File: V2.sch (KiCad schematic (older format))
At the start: 75 parts, among them J1 Input voltage, J20 Boot0, J21 Bed Temp, J22 Boot1, J26 USB_A, J27 LCD, J3 Bed Heater, J31 Bed level, J32 USB_B, J6 Head2, J7 Head1, M3 Motor Z2, M4 Motor Z1, M5 Motor Y, M6 Motor X, Q1 STN4NF20L, Q2 STN4NF20L, Q3 04N03LA, Q4 04N03LA, Q5 04N03LA, Q6 04N03LA, SW10 Button DOWN, SW11 Button UP, SW2 Boundary X, SW3 Boundary Y, SW4 Boundary Z1, SW5 Boundary Z2, SW6 Boundary E1, SW7 Boundary E2, SW8 Button BACK, SW9 Button OK, U1 LM2596S-5, U2 R-783.3-1.0, U3 STM32F105VCT6, U4 CP2104, Y1 hc49s

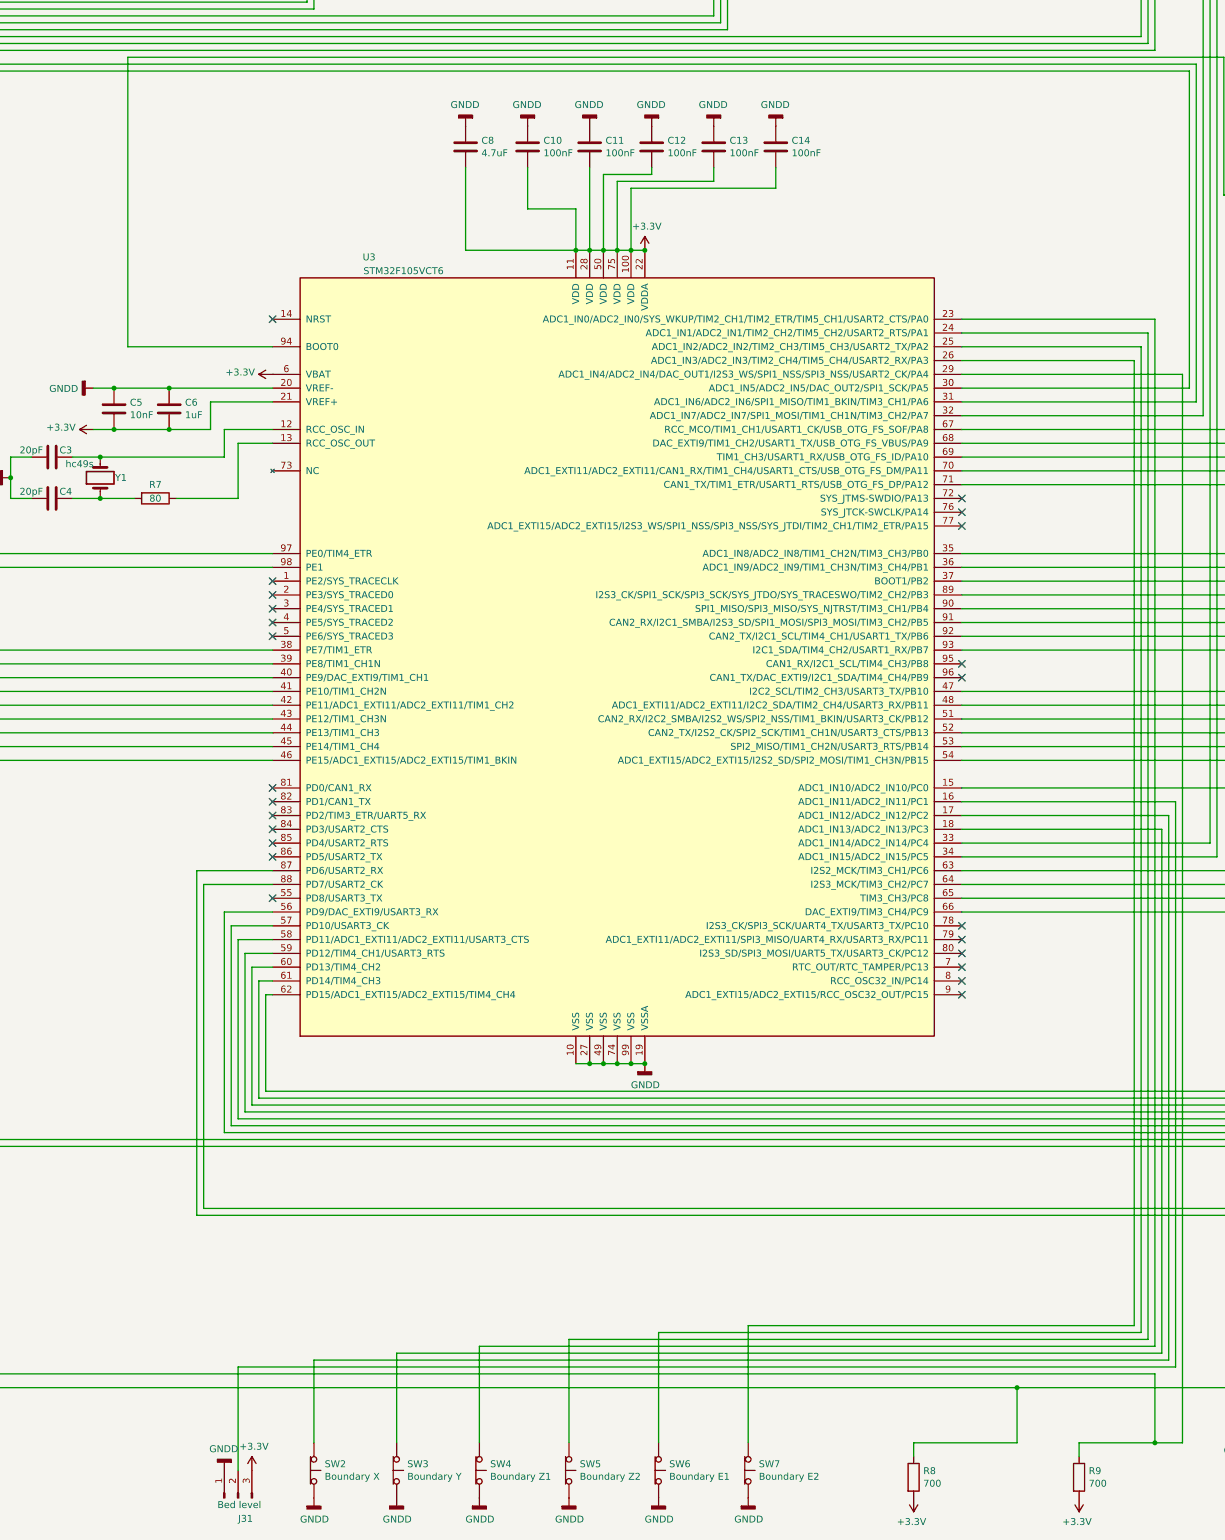
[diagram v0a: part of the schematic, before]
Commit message: Новая версия
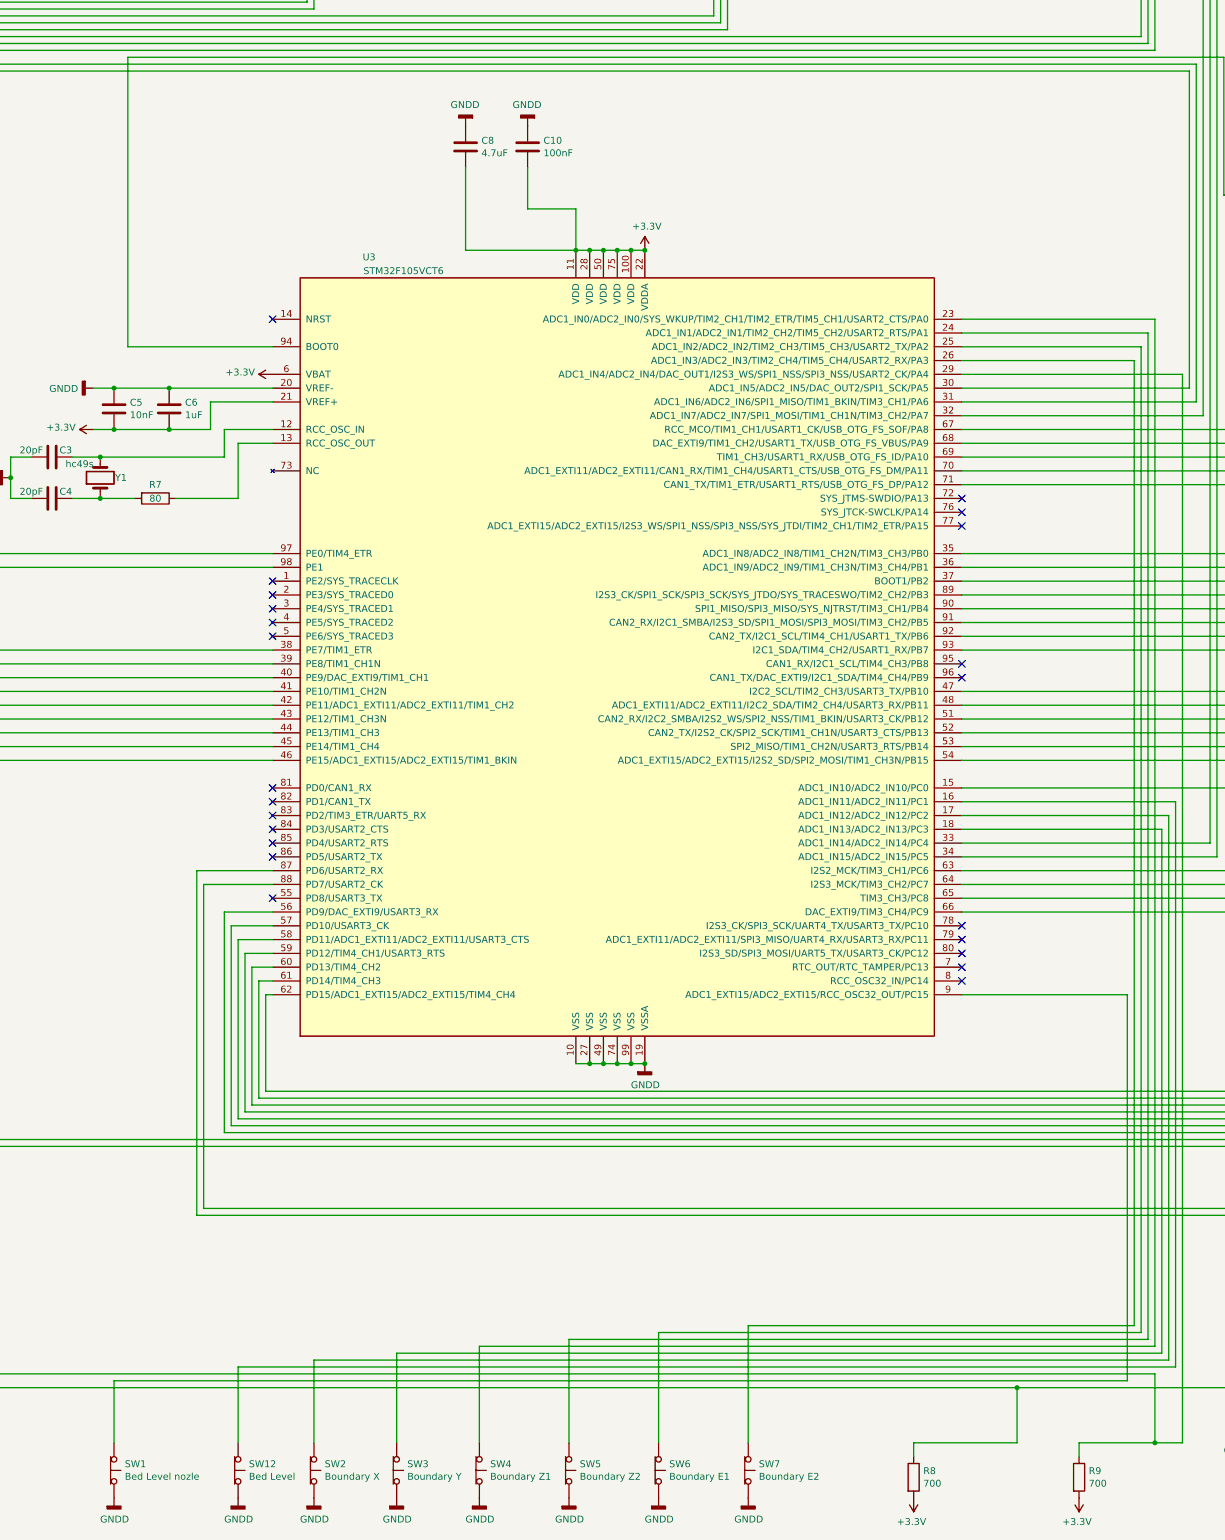
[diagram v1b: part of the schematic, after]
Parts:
- removed C11, C12, C13, C14: 100nF, Capacitor_SMD:C_1206_3216Metric, symbol V2-rescue:C-device
- removed J31: Bed level, Connector_PinHeader_2.54mm:PinHeader_1x03_P2.54mm_Vertical_SMD_Pin1Left, symbol V2-rescue:Conn_01x03_Male-Connector
- added SW1: Bed Level nozle, Connector_JST:JST_EH_B02B-EH-A_1x02_P2.50mm_Vertical, symbol V2-rescue:SW_Push_Open-Switch
- added SW12: Bed Level, Connector_JST:JST_EH_B02B-EH-A_1x02_P2.50mm_Vertical, symbol V2-rescue:SW_Push_Open-Switch
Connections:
- net GNDD: now also SW1.2 (B), SW12.2 (B)
- net at U3.16 (ADC1_IN11/ADC2_IN11/PC1): now also SW12.1 (A)
- net at U3.9 (ADC1_EXTI15/ADC2_EXTI15/RCC_OSC32_OUT/PC15): now also SW1.1 (A)
- no-connect marks 38 -> 37
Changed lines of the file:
@@
 EESchema Schematic File Version 4
 LIBS:V2-cache
-EELAYER 26 0
+EELAYER 29 0
 EELAYER END
 $Descr A2 23386 16535
@@
 $EndComp
 $Comp
-L V2-rescue:GNDD-power #PWR0130
-U 1 1 5C497D89
-P 8050 15550
-F 0 "#PWR0130" H 8050 15300 50  0001 C CNN
-F 1 "GNDD" H 8054 15395 50  0000 C CNN
-F 2 "" H 8050 15550 50  0001 C CNN
-F 3 "" H 8050 15550 50  0001 C CNN
-	1    8050 15550
-	-1   0    0    1
-$EndComp
-$Comp
 L V2-rescue:GNDD-power #PWR0131
 U 1 1 5C4985EB
@@
 	0    1    1    0
 $EndComp
-$Comp
-L V2-rescue:C-device C8
-U 1 1 5D0DBFC1
-P 9800 5950
-F 0 "C8" H 9915 5996 50  0000 L CNN
-F 1 "4.7uF" H 9915 5905 50  0000 L CNN
-F 2 "Capacitor_SMD:C_1206_3216Metric" H 9838 5800 50  0001 C CNN
-F 3 "" H 9800 5950 50  0001 C CNN
-	1    9800 5950
-	1    0    0    -1
-$EndComp
-$Comp
-L V2-rescue:GNDD-power #PWR0220
-U 1 1 5D0DC263
-P 9800 5800
-F 0 "#PWR0220" H 9800 5550 50  0001 C CNN
-F 1 "GNDD" H 9804 5645 50  0000 C CNN
-F 2 "" H 9800 5800 50  0001 C CNN
-F 3 "" H 9800 5800 50  0001 C CNN
-	1    9800 5800
-	-1   0    0    1
-$EndComp
-Wire Wire Line
-	10600 6700 10600 6400
-$Comp
-L V2-rescue:C-device C10
-U 1 1 5D18CD97
-P 10250 5950
-F 0 "C10" H 10365 5996 50  0000 L CNN
-F 1 "100nF" H 10365 5905 50  0000 L CNN
-F 2 "Capacitor_SMD:C_1206_3216Metric" H 10288 5800 50  0001 C CNN
-F 3 "" H 10250 5950 50  0001 C CNN
-	1    10250 5950
-	1    0    0    -1
-$EndComp
-$Comp
-L V2-rescue:C-device C11
-U 1 1 5D1B9492
-P 10700 5950
-F 0 "C11" H 10815 5996 50  0000 L CNN
-F 1 "100nF" H 10815 5905 50  0000 L CNN
-F 2 "Capacitor_SMD:C_1206_3216Metric" H 10738 5800 50  0001 C CNN
-F 3 "" H 10700 5950 50  0001 C CNN
-	1    10700 5950
-	1    0    0    -1
-$EndComp
-$Comp
-L V2-rescue:C-device C12
-U 1 1 5D1B9544
-P 11150 5950
-F 0 "C12" H 11265 5996 50  0000 L CNN
-F 1 "100nF" H 11265 5905 50  0000 L CNN
-F 2 "Capacitor_SMD:C_1206_3216Metric" H 11188 5800 50  0001 C CNN
-F 3 "" H 11150 5950 50  0001 C CNN
-	1    11150 5950
-	1    0    0    -1
-$EndComp
-$Comp
-L V2-rescue:C-device C13
-U 1 1 5D1B95F6
-P 11600 5950
-F 0 "C13" H 11715 5996 50  0000 L CNN
-F 1 "100nF" H 11715 5905 50  0000 L CNN
-F 2 "Capacitor_SMD:C_1206_3216Metric" H 11638 5800 50  0001 C CNN
-F 3 "" H 11600 5950 50  0001 C CNN
-	1    11600 5950
-	1    0    0    -1
-$EndComp
-$Comp
-L V2-rescue:C-device C14
-U 1 1 5D1B96B0
-P 12050 5950
-F 0 "C14" H 12165 5996 50  0000 L CNN
-F 1 "100nF" H 12165 5905 50  0000 L CNN
-F 2 "Capacitor_SMD:C_1206_3216Metric" H 12088 5800 50  0001 C CNN
-F 3 "" H 12050 5950 50  0001 C CNN
-	1    12050 5950
-	1    0    0    -1
-$EndComp
-Wire Wire Line
-	10600 6400 10250 6400
-Wire Wire Line
-	10250 6400 10250 6100
-Wire Wire Line
-	10700 6700 10700 6100
-Wire Wire Line
-	10800 6700 10800 6150
-Wire Wire Line
-	10800 6150 11150 6150
-Wire Wire Line
-	11150 6150 11150 6100
-Wire Wire Line
-	10900 6700 10900 6200
-Wire Wire Line
-	10900 6200 11600 6200
-Wire Wire Line
-	11600 6200 11600 6100
-Wire Wire Line
-	11000 6250 12050 6250
-Wire Wire Line
-	12050 6250 12050 6100
-Wire Wire Line
-	10600 6700 10700 6700
-Connection ~ 10600 6700
-Connection ~ 10700 6700
-Wire Wire Line
-	10700 6700 10800 6700
-Connection ~ 10800 6700
-Wire Wire Line
-	10800 6700 10900 6700
-Connection ~ 10900 6700
-Wire Wire Line
-	10900 6700 11000 6700
-Wire Wire Line
-	11000 6250 11000 6700
-Connection ~ 11000 6700
-Wire Wire Line
-	11000 6700 11100 6700
-Connection ~ 11100 6700
-Wire Wire Line
-	10600 6700 9800 6700
-Wire Wire Line
-	9800 6700 9800 6100
-$Comp
-L V2-rescue:GNDD-power #PWR0221
-U 1 1 5D4196BD
-P 10250 5800
-F 0 "#PWR0221" H 10250 5550 50  0001 C CNN
-F 1 "GNDD" H 10254 5645 50  0000 C CNN
-F 2 "" H 10250 5800 50  0001 C CNN
-F 3 "" H 10250 5800 50  0001 C CNN
-	1    10250 5800
-	-1   0    0    1
-$EndComp
-$Comp
-L V2-rescue:GNDD-power #PWR0222
-U 1 1 5D419762
-P 10700 5800
-F 0 "#PWR0222" H 10700 5550 50  0001 C CNN
-F 1 "GNDD" H 10704 5645 50  0000 C CNN
-F 2 "" H 10700 5800 50  0001 C CNN
-F 3 "" H 10700 5800 50  0001 C CNN
-	1    10700 5800
-	-1   0    0    1
-$EndComp
-$Comp
-L V2-rescue:GNDD-power #PWR0223
-U 1 1 5D419807
-P 11150 5800
-F 0 "#PWR0223" H 11150 5550 50  0001 C CNN
-F 1 "GNDD" H 11154 5645 50  0000 C CNN
-F 2 "" H 11150 5800 50  0001 C CNN
-F 3 "" H 11150 5800 50  0001 C CNN
-	1    11150 5800
-	-1   0    0    1
-$EndComp
-$Comp
-L V2-rescue:GNDD-power #PWR0224
-U 1 1 5D4198AC
-P 11600 5800
-F 0 "#PWR0224" H 11600 5550 50  0001 C CNN
-F 1 "GNDD" H 11604 5645 50  0000 C CNN
-F 2 "" H 11600 5800 50  0001 C CNN
-F 3 "" H 11600 5800 50  0001 C CNN
-	1    11600 5800
-	-1   0    0    1
-$EndComp
-$Comp
-L V2-rescue:GNDD-power #PWR0225
-U 1 1 5D419951
-P 12050 5800
-F 0 "#PWR0225" H 12050 5550 50  0001 C CNN
-F 1 "GNDD" H 12054 5645 50  0000 C CNN
-F 2 "" H 12050 5800 50  0001 C CNN
-F 3 "" H 12050 5800 50  0001 C CNN
-	1    12050 5800
-	-1   0    0    1
-$EndComp
 Wire Wire Line
 	10600 12600 10700 12600
@@
 	7350 7400 8400 7400
 NoConn ~ 8400 7200
-NoConn ~ 13400 12100
 Wire Wire Line
 	4300 4550 4300 4500
@@
 $EndComp
 $Comp
-L V2-rescue:Conn_01x03_Male-Connector J31
-U 1 1 5C6206CB
-P 8150 15750
-F 0 "J31" V 8000 15750 50  0000 R CNN
-F 1 "Bed level" V 8100 15900 50  0000 R CNN
-F 2 "Connector_PinHeader_2.54mm:PinHeader_1x03_P2.54mm_Vertical_SMD_Pin1Left" H 8150 15750 50  0001 C CNN
-F 3 "~" H 8150 15750 50  0001 C CNN
-	1    8150 15750
-	0    -1   -1   0
-$EndComp
-$Comp
-L V2-rescue:+3.3V-power #PWR0241
-U 1 1 5C789638
-P 8250 15550
-F 0 "#PWR0241" H 8250 15400 50  0001 C CNN
-F 1 "+3.3V" H 8265 15723 50  0000 C CNN
-F 2 "" H 8250 15550 50  0001 C CNN
-F 3 "" H 8250 15550 50  0001 C CNN
-	1    8250 15550
-	1    0    0    -1
-$EndComp
-$Comp
 L POWER_LIB:PWR_FLAG #FLG0101
 U 1 1 5C534BEB
@@
 	14950 14800 8150 14800
 Wire Wire Line
-	8150 14800 8150 15550
-Wire Wire Line
 	8700 15350 8700 14750
 Wire Wire Line
@@
 Wire Wire Line
 	14650 7500 13400 7500
+$Comp
+L V2-rescue:GNDD-power #PWR0130
+U 1 1 5C497D89
+P 8150 15750
+F 0 "#PWR0130" H 8150 15500 50  0001 C CNN
+F 1 "GNDD" H 8154 15595 50  0000 C CNN
+F 2 "" H 8150 15750 50  0001 C CNN
+F 3 "" H 8150 15750 50  0001 C CNN
+	1    8150 15750
+	1    0    0    -1
+$EndComp
+$Comp
+L V2-rescue:SW_Push_Open-Switch SW12
+U 1 1 5CFCCBD5
+P 8150 15550
+F 0 "SW12" V 8104 15628 50  0000 L CNN
+F 1 "Bed Level" V 8195 15628 50  0000 L CNN
+F 2 "Connector_JST:JST_EH_B02B-EH-A_1x02_P2.50mm_Vertical" H 8150 15750 50  0001 C CNN
+F 3 "" H 8150 15750 50  0001 C CNN
+	1    8150 15550
+	0    1    1    0
+$EndComp
+Wire Wire Line
+	8150 14800 8150 15350
+$Comp
+L V2-rescue:SW_Push_Open-Switch SW1
+U 1 1 5D0AFB29
+P 7250 15550
+F 0 "SW1" V 7204 15628 50  0000 L CNN
+F 1 "Bed Level nozle" V 7295 15628 50  0000 L CNN
+F 2 "Connector_JST:JST_EH_B02B-EH-A_1x02_P2.50mm_Vertical" H 7250 15750 50  0001 C CNN
+F 3 "" H 7250 15750 50  0001 C CNN
+	1    7250 15550
+	0    1    1    0
+$EndComp
+$Comp
+L V2-rescue:GNDD-power #PWR0114
+U 1 1 5D0B183C
+P 7250 15750
+F 0 "#PWR0114" H 7250 15500 50  0001 C CNN
+F 1 "GNDD" H 7254 15595 50  0000 C CNN
+F 2 "" H 7250 15750 50  0001 C CNN
+F 3 "" H 7250 15750 50  0001 C CNN
+	1    7250 15750
+	1    0    0    -1
+$EndComp
+Wire Wire Line
+	13400 12100 14600 12100
+Wire Wire Line
+	14600 12100 14600 14900
+Wire Wire Line
+	14600 14900 7250 14900
+Wire Wire Line
+	7250 14900 7250 15350
+Connection ~ 11100 6700
+Wire Wire Line
+	11000 6700 11100 6700
+Connection ~ 11000 6700
+Wire Wire Line
+	10900 6700 11000 6700
+Connection ~ 10900 6700
+Wire Wire Line
+	10800 6700 10900 6700
+Connection ~ 10800 6700
+Wire Wire Line
+	10700 6700 10800 6700
+Connection ~ 10700 6700
+Wire Wire Line
+	10600 6700 10700 6700
+Connection ~ 10600 6700
+Wire Wire Line
+	10600 6700 9800 6700
+Wire Wire Line
+	10600 6700 10600 6400
+Wire Wire Line
+	10600 6400 10250 6400
+Wire Wire Line
+	9800 6700 9800 6100
+Wire Wire Line
+	10250 6400 10250 6100
+$Comp
+L V2-rescue:C-device C10
+U 1 1 5D18CD97
+P 10250 5950
+F 0 "C10" H 10365 5996 50  0000 L CNN
+F 1 "100nF" H 10365 5905 50  0000 L CNN
+F 2 "Capacitor_SMD:C_1206_3216Metric" H 10288 5800 50  0001 C CNN
+F 3 "" H 10250 5950 50  0001 C CNN
+	1    10250 5950
+	1    0    0    -1
+$EndComp
+$Comp
+L V2-rescue:GNDD-power #PWR0221
+U 1 1 5D4196BD
+P 10250 5800
+F 0 "#PWR0221" H 10250 5550 50  0001 C CNN
+F 1 "GNDD" H 10254 5645 50  0000 C CNN
+F 2 "" H 10250 5800 50  0001 C CNN
+F 3 "" H 10250 5800 50  0001 C CNN
+	1    10250 5800
+	-1   0    0    1
+$EndComp
+$Comp
+L V2-rescue:GNDD-power #PWR0220
+U 1 1 5D0DC263
+P 9800 5800
+F 0 "#PWR0220" H 9800 5550 50  0001 C CNN
+F 1 "GNDD" H 9804 5645 50  0000 C CNN
+F 2 "" H 9800 5800 50  0001 C CNN
+F 3 "" H 9800 5800 50  0001 C CNN
+	1    9800 5800
+	-1   0    0    1
+$EndComp
+$Comp
+L V2-rescue:C-device C8
+U 1 1 5D0DBFC1
+P 9800 5950
+F 0 "C8" H 9915 5996 50  0000 L CNN
+F 1 "4.7uF" H 9915 5905 50  0000 L CNN
+F 2 "Capacitor_SMD:C_1206_3216Metric" H 9838 5800 50  0001 C CNN
+F 3 "" H 9800 5950 50  0001 C CNN
+	1    9800 5950
+	1    0    0    -1
+$EndComp
 $EndSCHEMATC
